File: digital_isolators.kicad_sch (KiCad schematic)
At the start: 9 parts, among them U4 ISO7760DBQ, U5 ISO7760DBQ, U6 ISO7760DBQ

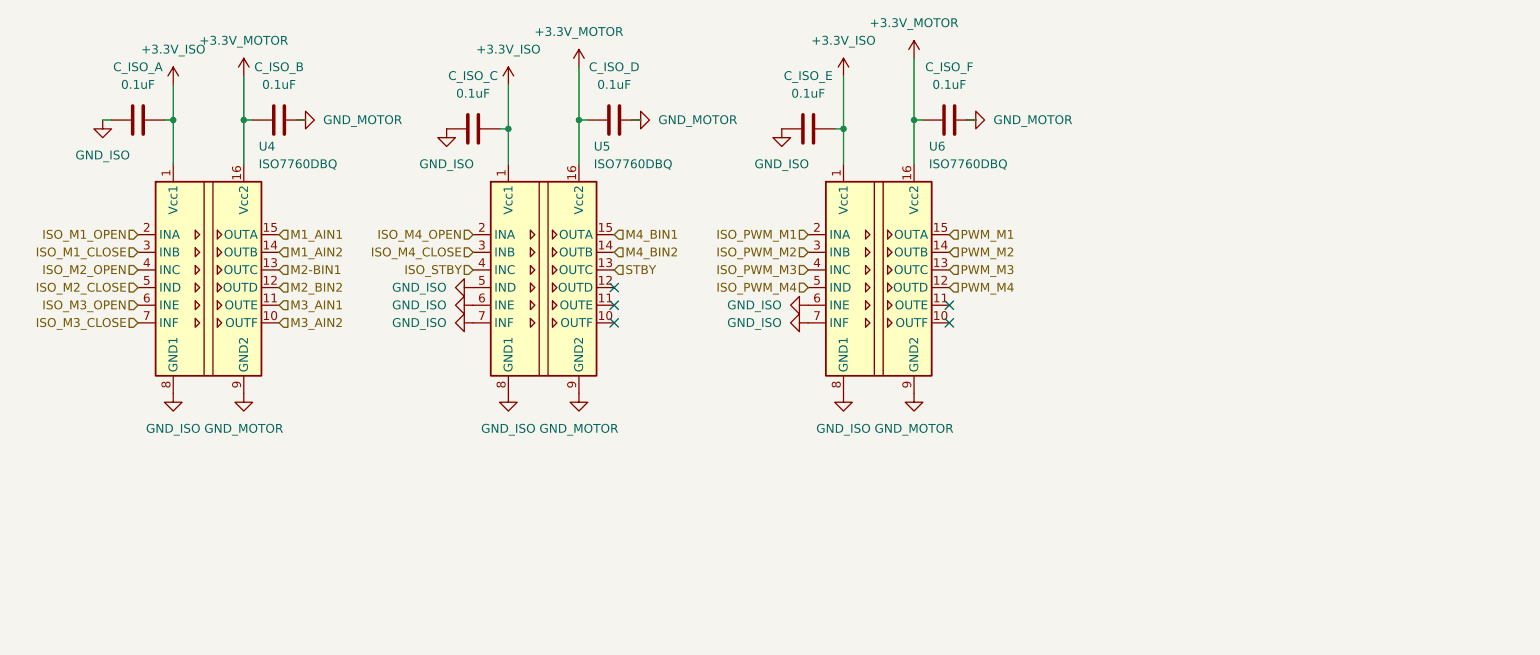
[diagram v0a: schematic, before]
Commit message: Started running traces
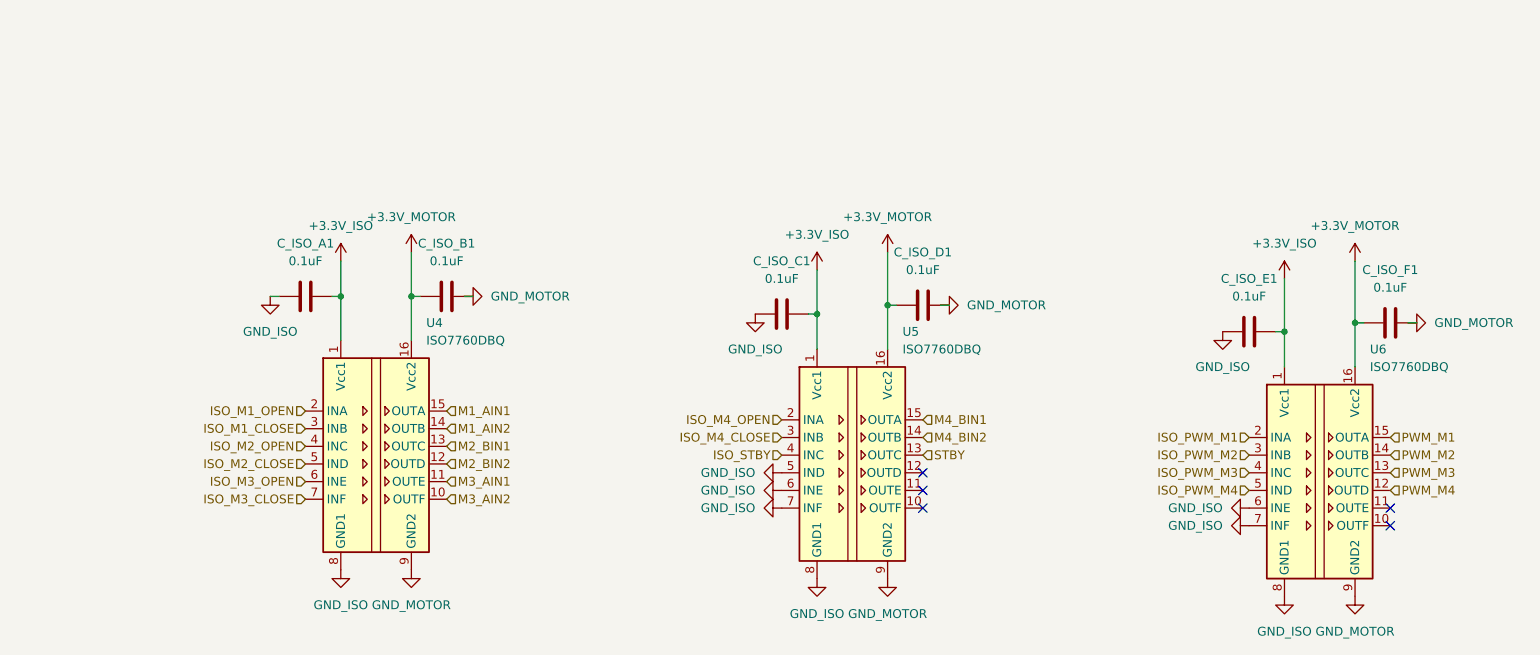
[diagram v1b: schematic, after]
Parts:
- C_ISO_A1: renamed from C_ISO_A; footprint (none) -> Capacitor_SMD:C_0603_1608Metric
- C_ISO_B1: renamed from C_ISO_B; footprint (none) -> Capacitor_SMD:C_0603_1608Metric
- C_ISO_C1: renamed from C_ISO_C; footprint (none) -> Capacitor_SMD:C_0603_1608Metric
- C_ISO_D1: renamed from C_ISO_D; footprint (none) -> Capacitor_SMD:C_0603_1608Metric
- C_ISO_E1: renamed from C_ISO_E; footprint (none) -> Capacitor_SMD:C_0603_1608Metric
- C_ISO_F1: renamed from C_ISO_F; footprint (none) -> Capacitor_SMD:C_0603_1608Metric
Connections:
- net M2-BIN1 renamed M2_BIN1
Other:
- moved on the sheet: C_ISO_A1, C_ISO_B1, C_ISO_C1, C_ISO_D1, C_ISO_E1, C_ISO_F1, U4, U5, U6
